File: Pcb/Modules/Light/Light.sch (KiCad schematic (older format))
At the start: 9 parts, among them J1 JACK_RJ45, J2 JACK_STEREO, Q1 TEPT4400, Q2 Q_NMOS_GSD

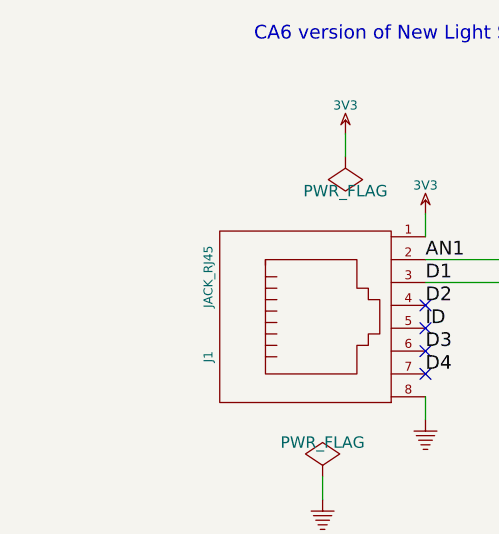
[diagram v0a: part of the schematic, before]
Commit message: Update pcbs
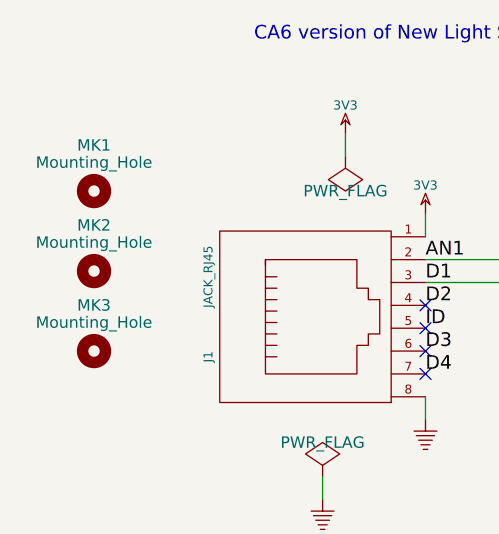
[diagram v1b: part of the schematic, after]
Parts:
- added MK1, MK2, MK3: Mounting_Hole, Mounting_Holes:MountingHole_2.5mm_Pad, symbol Mounting_Hole
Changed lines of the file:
@@
 LIBS:zetex
 LIBS:Zilog
+LIBS:Light-cache
 EELAYER 25 0
 EELAYER END
@@
 	1    0    0    -1
 $EndComp
+$Comp
+L Mounting_Hole MK1
+U 1 1 5A1F1815
+P 3200 3100
+F 0 "MK1" H 3200 3300 50  0000 C CNN
+F 1 "Mounting_Hole" H 3200 3225 50  0000 C CNN
+F 2 "Mounting_Holes:MountingHole_2.5mm_Pad" H 3200 3100 60  0001 C CNN
+F 3 "" H 3200 3100 60  0001 C CNN
+	1    3200 3100
+	1    0    0    -1
+$EndComp
+$Comp
+L Mounting_Hole MK2
+U 1 1 5A1F1870
+P 3200 3450
+F 0 "MK2" H 3200 3650 50  0000 C CNN
+F 1 "Mounting_Hole" H 3200 3575 50  0000 C CNN
+F 2 "Mounting_Holes:MountingHole_2.5mm_Pad" H 3200 3450 60  0001 C CNN
+F 3 "" H 3200 3450 60  0001 C CNN
+	1    3200 3450
+	1    0    0    -1
+$EndComp
+$Comp
+L Mounting_Hole MK3
+U 1 1 5A1F18E3
+P 3200 3800
+F 0 "MK3" H 3200 4000 50  0000 C CNN
+F 1 "Mounting_Hole" H 3200 3925 50  0000 C CNN
+F 2 "Mounting_Holes:MountingHole_2.5mm_Pad" H 3200 3800 60  0001 C CNN
+F 3 "" H 3200 3800 60  0001 C CNN
+	1    3200 3800
+	1    0    0    -1
+$EndComp
